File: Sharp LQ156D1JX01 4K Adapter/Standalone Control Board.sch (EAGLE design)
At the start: 1 part

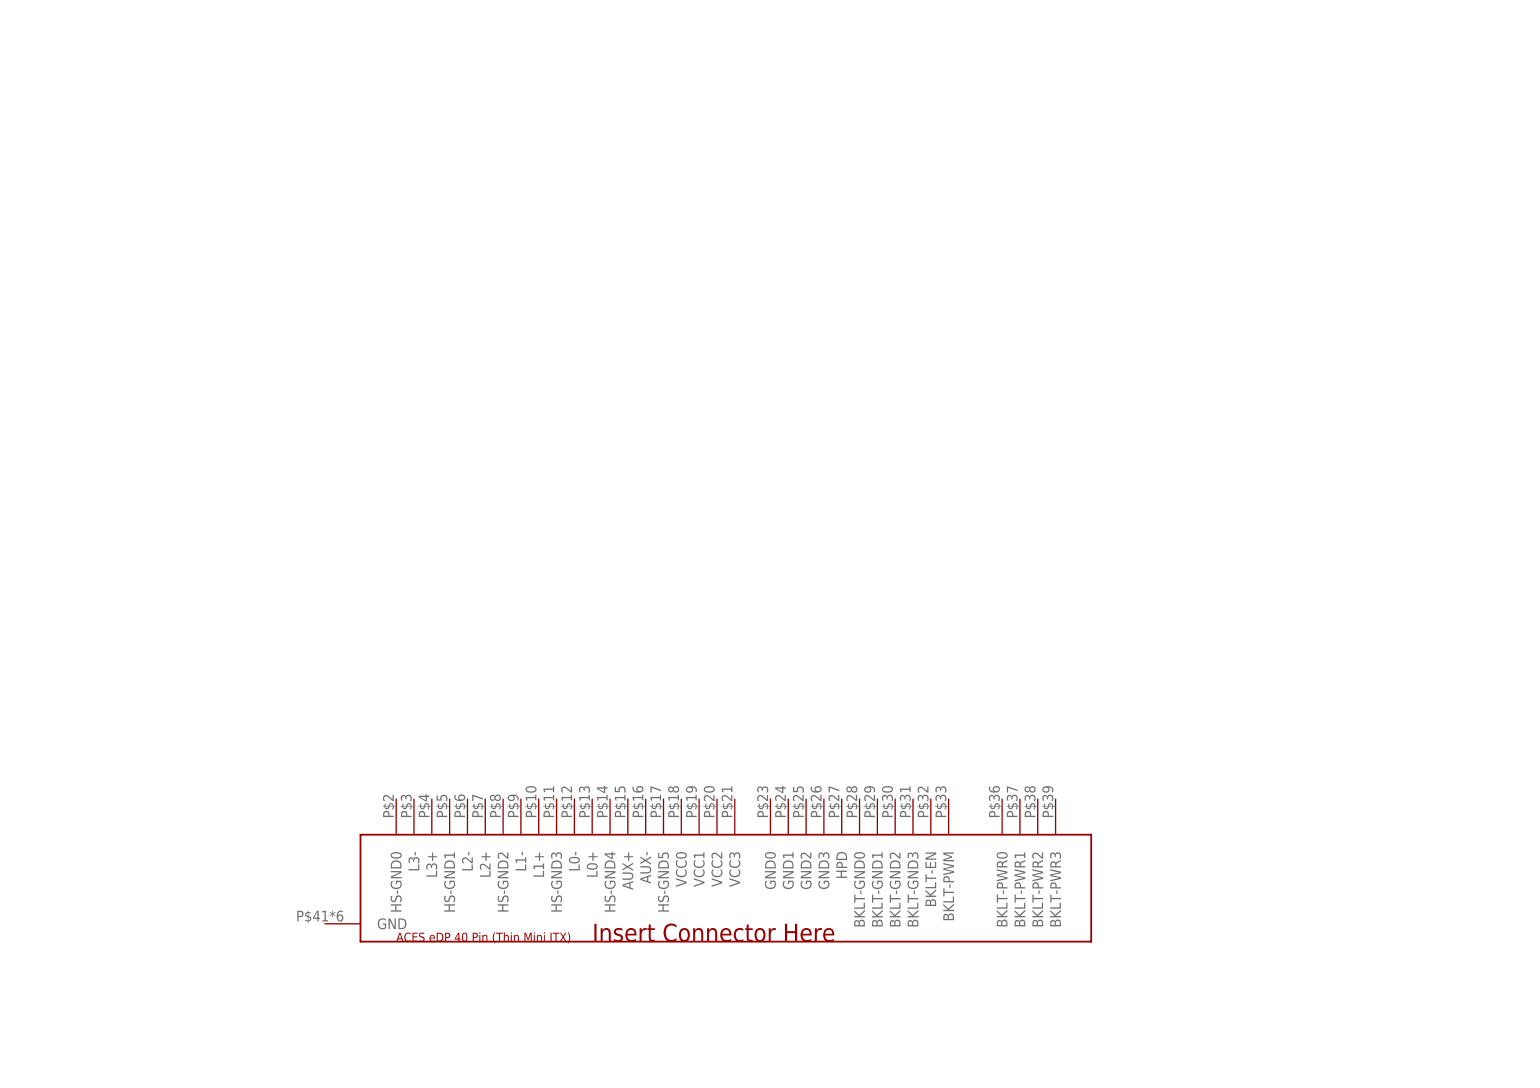
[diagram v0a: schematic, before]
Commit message: Working on sharp 4k. so many k's
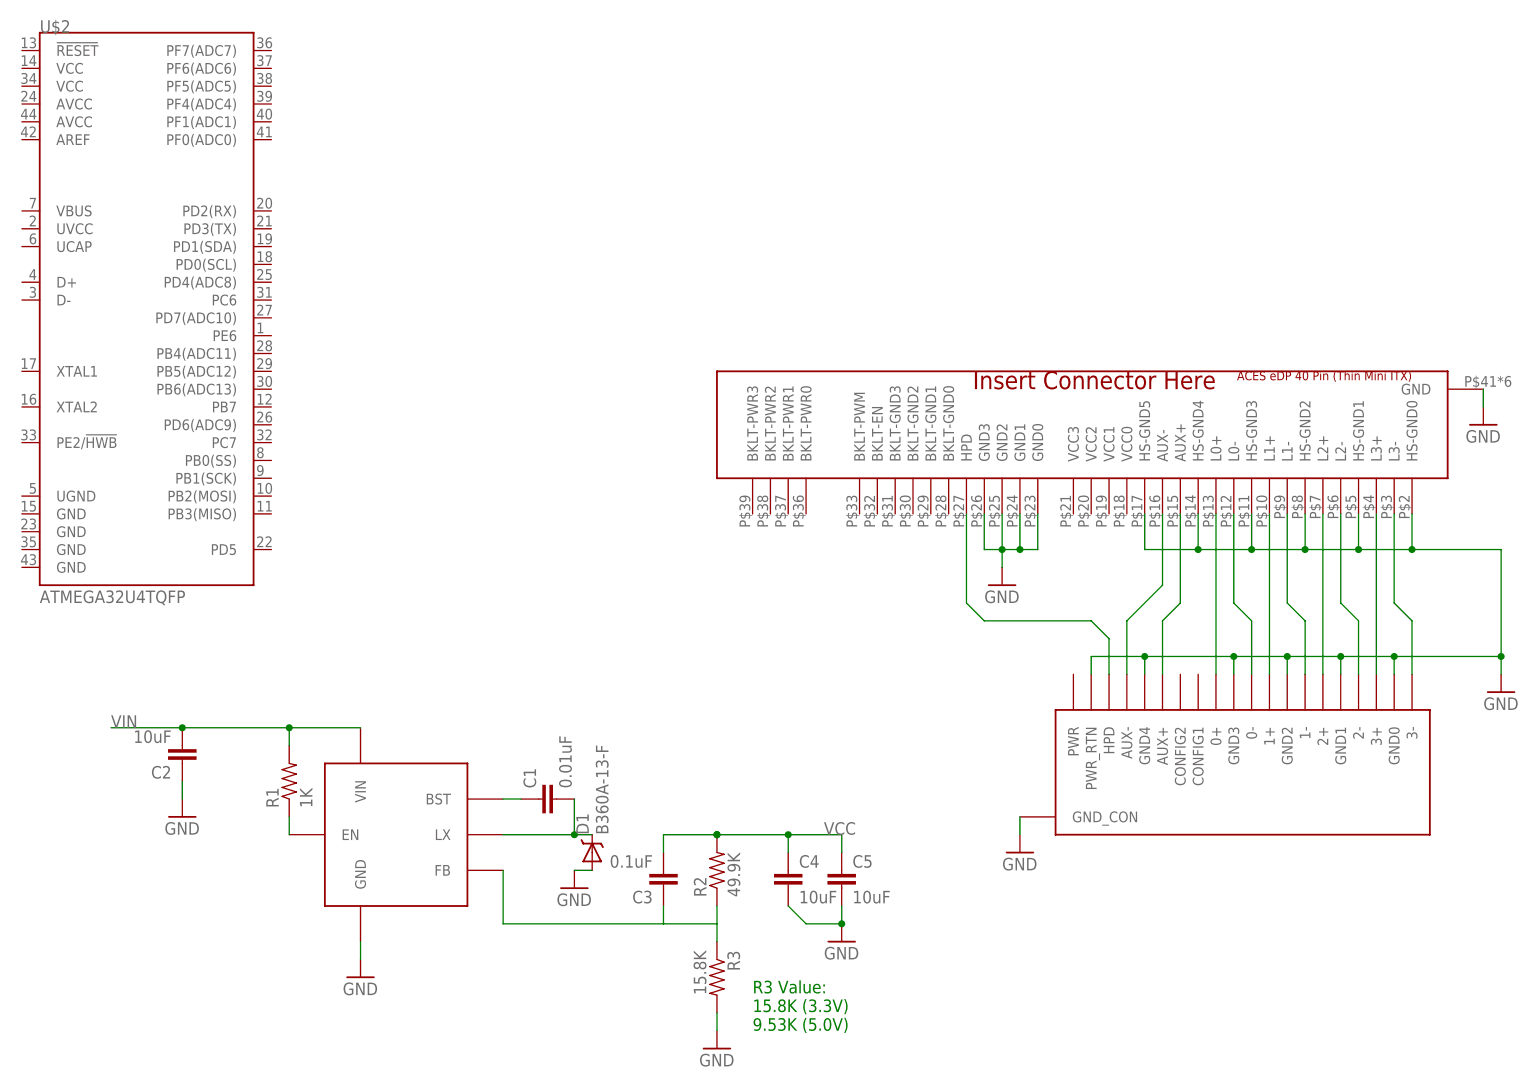
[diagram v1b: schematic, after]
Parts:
- added C1: 0.01uF, SparkFun-Passives:CAP0805
- added C2, C4, C5: 10uF, SparkFun-Passives:CAP0805
- added C3: 0.1uF, SparkFun-Passives:CAP0805
- added D1: B360A-13-F, SparkFun-DiscreteSemi:DIODE-SCHOTTKY_
- added R1: 1K, SparkFun-Passives:RESISTOR0805-RES
- added R2: 49.9K, SparkFun-Passives:RESISTOR0805-RES
- added R3: 15.8K, SparkFun-Passives:RESISTOR0805-RES
- added U$1: DP-SINK, LCD Connectors:DP-SINK
- added U$2: ATMEGA32U4TQFP, SparkFun-DigitalIC:ATMEGA32U4TQFP
- added U$3: AOZ1281-BUCK, LCD Connectors:AOZ1281-BUCK
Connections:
- new net 0_N: F1.L0-, U$1.0-
- new net 0_P: F1.L0+, U$1.0+
- new net 1_N: F1.L1-, U$1.1-
- new net 1_P: F1.L1+, U$1.1+
- new net 2_N: F1.L2-, U$1.2-
- new net 2_P: F1.L2+, U$1.2+
- new net 3_N: F1.L3-, U$1.3-
- new net 3_P: F1.L3+, U$1.3+
- new net AUX_N: F1.AUX-, U$1.AUX-
- new net AUX_P: F1.AUX+, U$1.AUX+
- new net GND: C2.1, C4.2, C5.2, D1.A, F1.GND, F1.GND0, F1.GND1, F1.GND2, F1.GND3, F1.HS-GND0, F1.HS-GND1, F1.HS-GND2, F1.HS-GND3, F1.HS-GND4, F1.HS-GND5, R3.2, U$1.GND0, U$1.GND1, U$1.GND2, U$1.GND3, U$1.GND4, U$1.GND_CON, U$1.PWR_RTN, U$3.GND
- new net N$1: R1.1, U$3.EN
- new net N$14: F1.HPD, U$1.HPD
- new net N$2: C3.1, U$3.FB
- new net N$3: C1.1, U$3.BST
- new net N$4: C1.2, D1.C, U$3.LX
- new net N$5: R2.1, R3.1
- new net VCC: C3.2, C4.1, C5.1, R2.2
- new net VIN: C2.2, R1.2, U$3.VIN
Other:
- note added: "R3 Value: 15.8K (3.3V) 9.53K (5.0V)"
